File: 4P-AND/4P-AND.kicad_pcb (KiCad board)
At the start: 2 copper layers, 50.2 x 18.4 mm, 10 parts, among them J1 Conn_01x02, J2 Conn_01x02, J3 Conn_01x02, J4 Conn_01x02

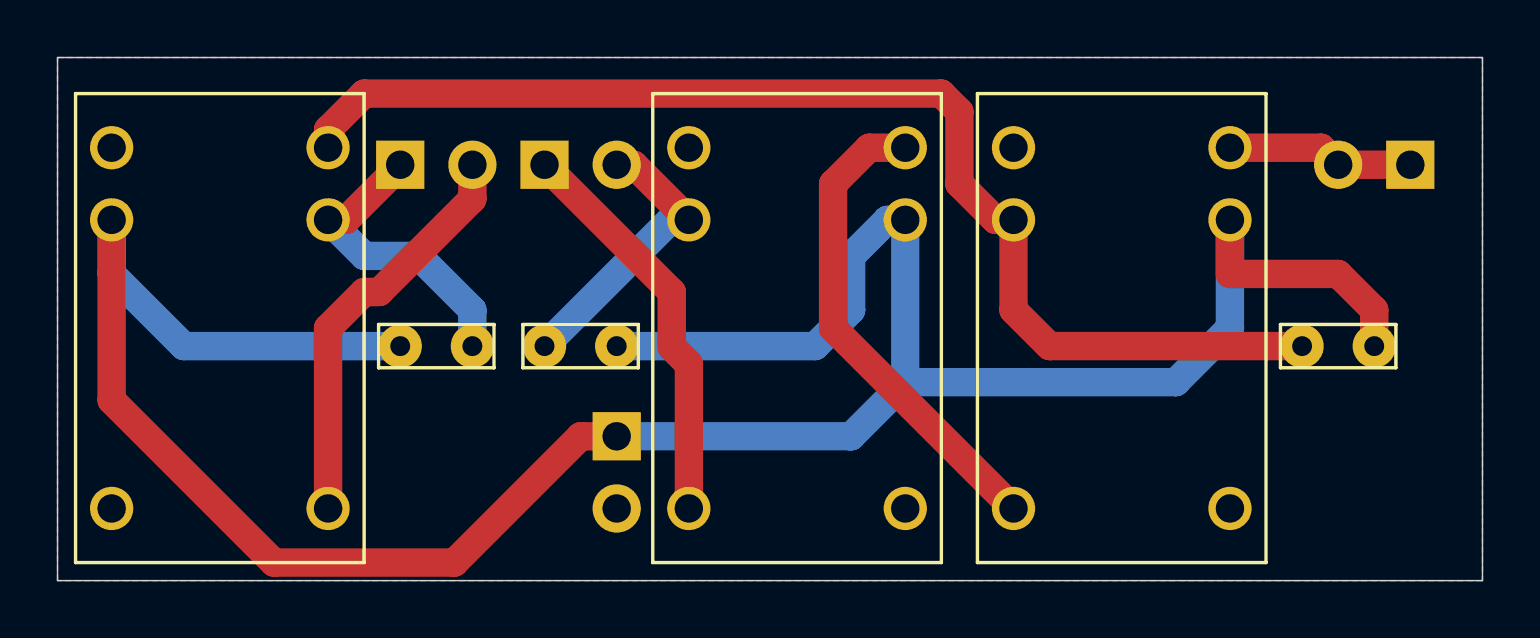
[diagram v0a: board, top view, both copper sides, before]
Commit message: Add files via upload
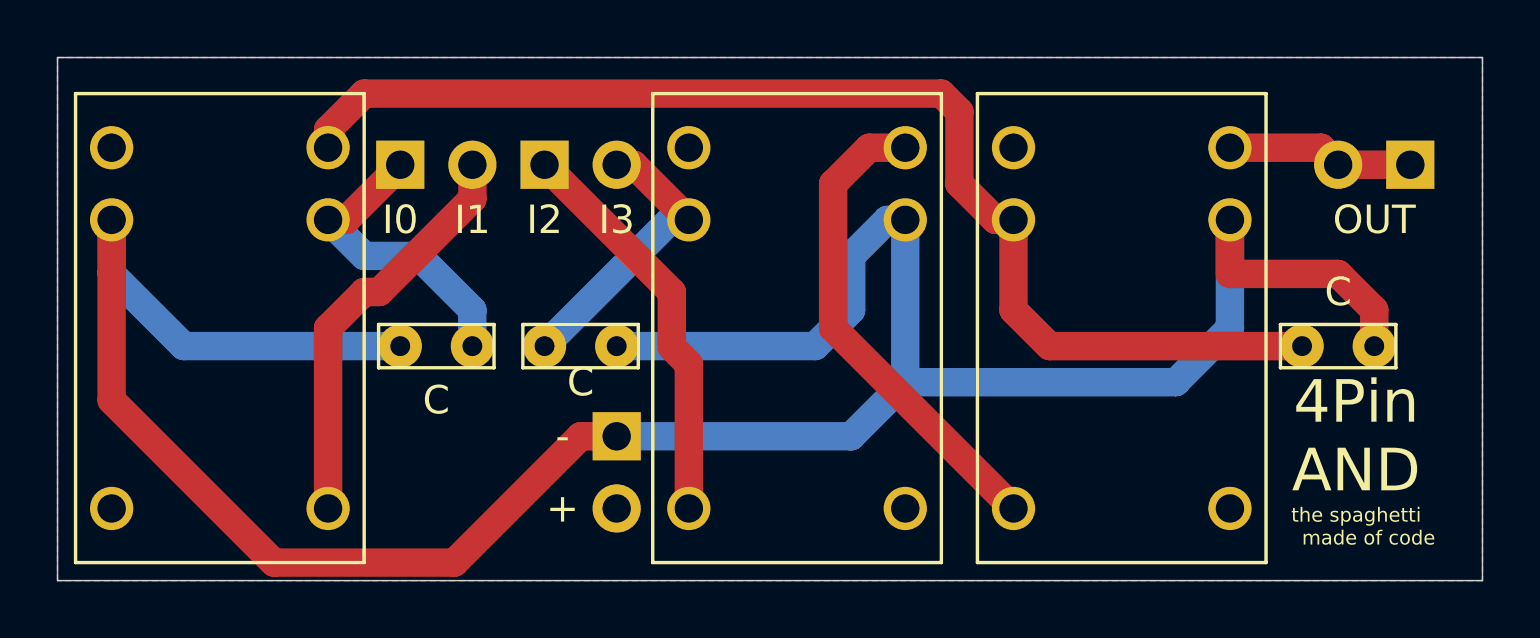
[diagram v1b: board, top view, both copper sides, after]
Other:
- board text added: "+"
- board text added: "-"
- board text added: "4Pin AND"
- board text added: "C"
- board text added: "I0"
- board text added: "I1"
- board text added: "I2"
- board text added: "I3"
- board text added: "OUT"
- board text added: "the spaghetti made of code"
